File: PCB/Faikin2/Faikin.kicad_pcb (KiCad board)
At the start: 2 copper layers, 70 x 70 mm, 33 parts, among them J1 1x5, J3 Shelly, Q1 BSS138PS, U2 Barcode, U3 MD8942, U4 ESP32-S3-MINI-1

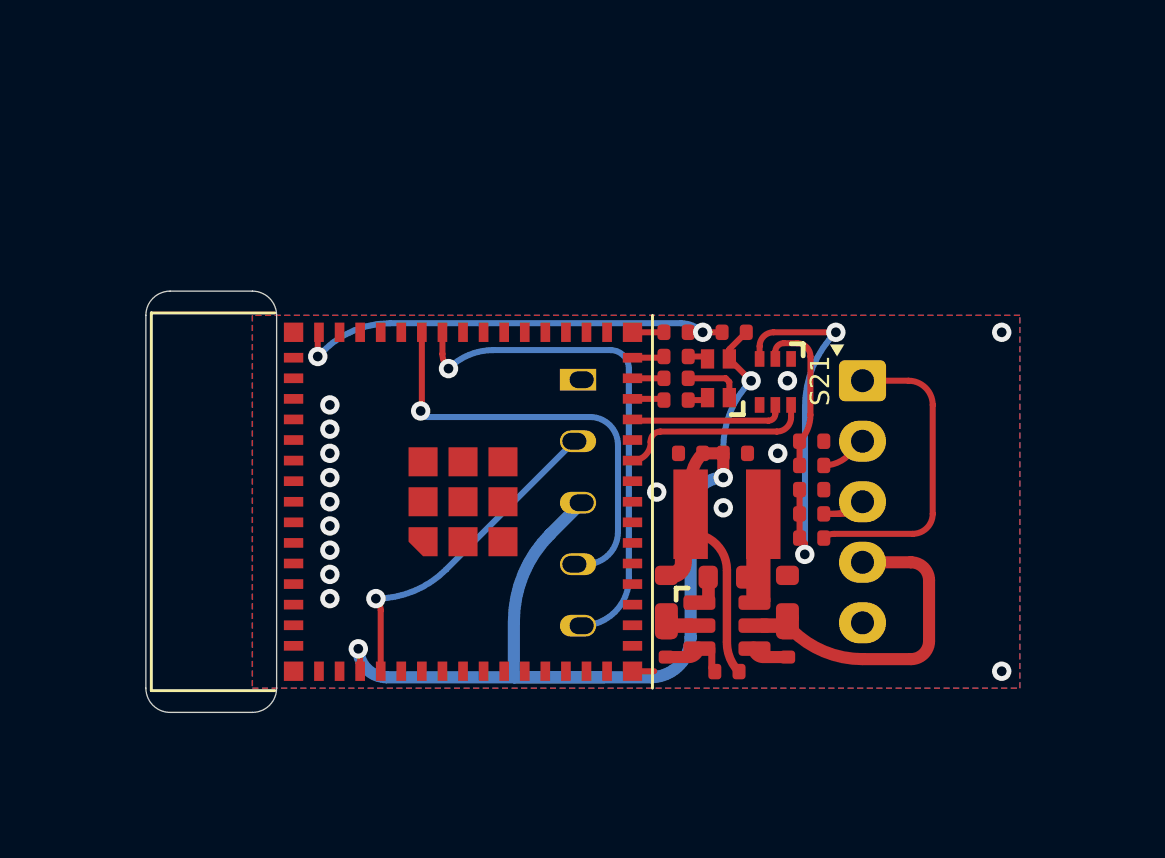
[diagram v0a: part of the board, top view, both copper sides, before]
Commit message: Adjusted for panel and barcode
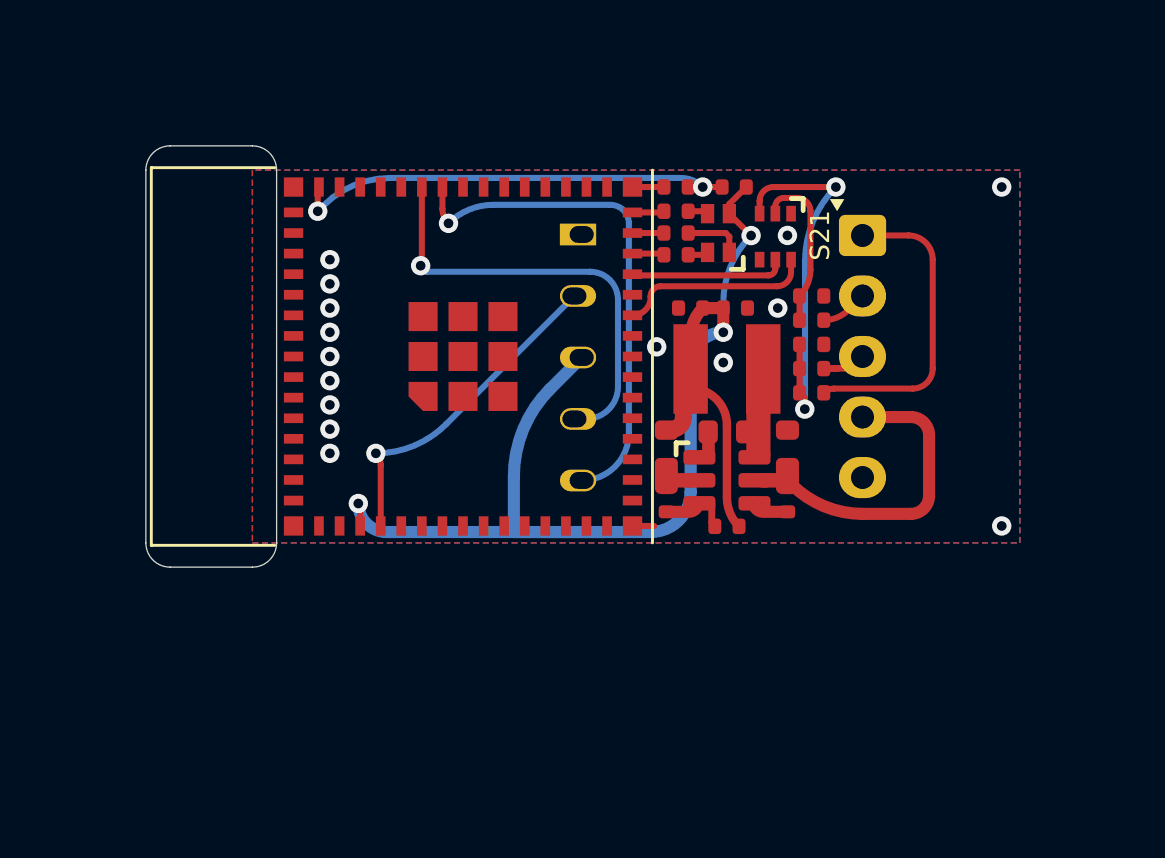
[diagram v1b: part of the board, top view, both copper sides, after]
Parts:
- moved R10 6.00 mm to (137.5, 60.9)
- moved R11 6.00 mm to (142.5, 60.9)
- moved C2 6.00 mm to (138.5, 53.0)
- moved C3 6.00 mm to (143.5, 54.5)
- moved C4 6.00 mm to (143.5, 52.5)
- moved C5 6.00 mm to (140.3, 53.0)
- moved C6 6.00 mm to (137.9, 48.0)
- moved C8 6.00 mm to (142.5, 58.8)
- moved C9 6.00 mm to (137.5, 58.8)
- moved D2 6.00 mm to (139.7, 49.9)
- moved J1 6.00 mm to (145.6, 50.0)
- moved J3 6.00 mm to (133.8, 55.0)
- moved L2 6.00 mm to (140.0, 55.5)
- moved Q1 6.00 mm to (142.0, 50.0)
- moved R1 6.00 mm to (143.5, 56.5)
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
